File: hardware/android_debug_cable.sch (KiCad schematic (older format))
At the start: 11 parts, among them P1 USB_OTG, P2 50-00397, P3 CONN_01X04, U1 TCR2EF18, U2 CP2102N-A01-GQFN24

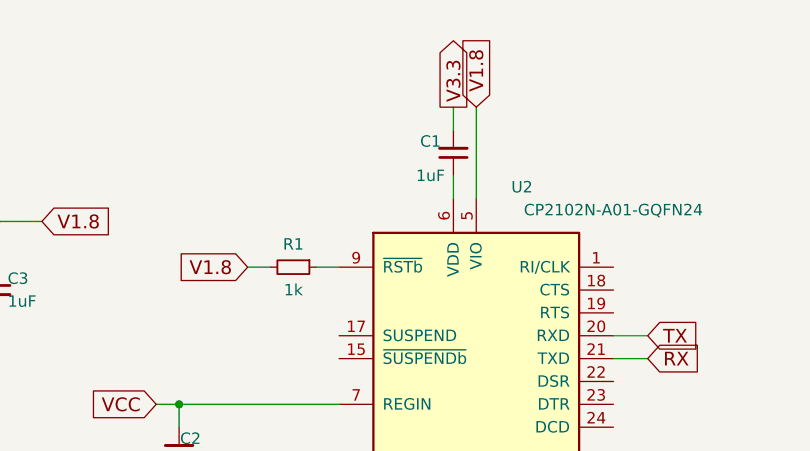
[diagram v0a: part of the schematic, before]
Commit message: v0.6
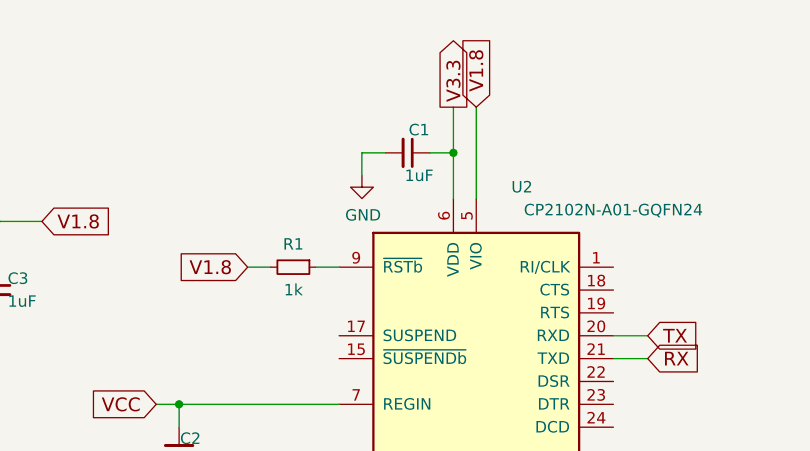
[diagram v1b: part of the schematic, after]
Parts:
- C1: footprint Capacitors_SMD:C_0402 -> (none)
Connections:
- net GND: now also C1.2
- net V3.3: now also C1.1, U2.6 (VDD); no longer C1.2
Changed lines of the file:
@@
 V1.8
-$Comp
-L C_Small C1
-U 1 1 57AE72A2
-P 5550 2650
-F 0 "C1" H 5650 2600 50  0000 C CNN
-F 1 "1uF" H 5650 2750 50  0000 C CNN
-F 2 "Capacitors_SMD:C_0402" H 5550 2650 50  0001 C CNN
-F 3 "" H 5550 2650 50  0000 C CNN
-	1    5550 2650
-	-1   0    0    1
-$EndComp
 $Comp
 L C_Small C2
@@
 	4250 3750 5050 3750
 Wire Wire Line
-	5550 2750 5550 2850
-Wire Wire Line
-	5550 2550 5550 2450
+	5550 2450 5550 2850
 Wire Wire Line
 	5050 3150 4950 3150
@@
 Wire Wire Line
 	4350 3850 4350 3750
+$Comp
+L C_Small C1
+U 1 1 59579678
+P 5350 2650
+F 0 "C1" V 5250 2700 50  0000 C CNN
+F 1 "1uF" V 5450 2700 50  0000 C CNN
+F 2 "" H 5350 2650 50  0001 C CNN
+F 3 "" H 5350 2650 50  0001 C CNN
+	1    5350 2650
+	0    1    1    0
+$EndComp
+Wire Wire Line
+	5450 2650 5550 2650
+Connection ~ 5550 2650
+$Comp
+L GND #PWR?
+U 1 1 595798C6
+P 5150 2750
+F 0 "#PWR?" H 5150 2500 50  0001 C CNN
+F 1 "GND" H 5155 2577 50  0000 C CNN
+F 2 "" H 5150 2750 50  0001 C CNN
+F 3 "" H 5150 2750 50  0001 C CNN
+	1    5150 2750
+	1    0    0    -1
+$EndComp
+Wire Wire Line
+	5150 2750 5150 2650
+Wire Wire Line
+	5150 2650 5250 2650
 $EndSCHEMATC
